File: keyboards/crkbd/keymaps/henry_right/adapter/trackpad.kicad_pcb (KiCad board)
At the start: 2 copper layers, 33.4 x 18.4 mm, 9 parts, among them J1 Conn_01x12, U1 Elite-C, U3 NCP1117-3.3_SOT223, U4 TXB0104D

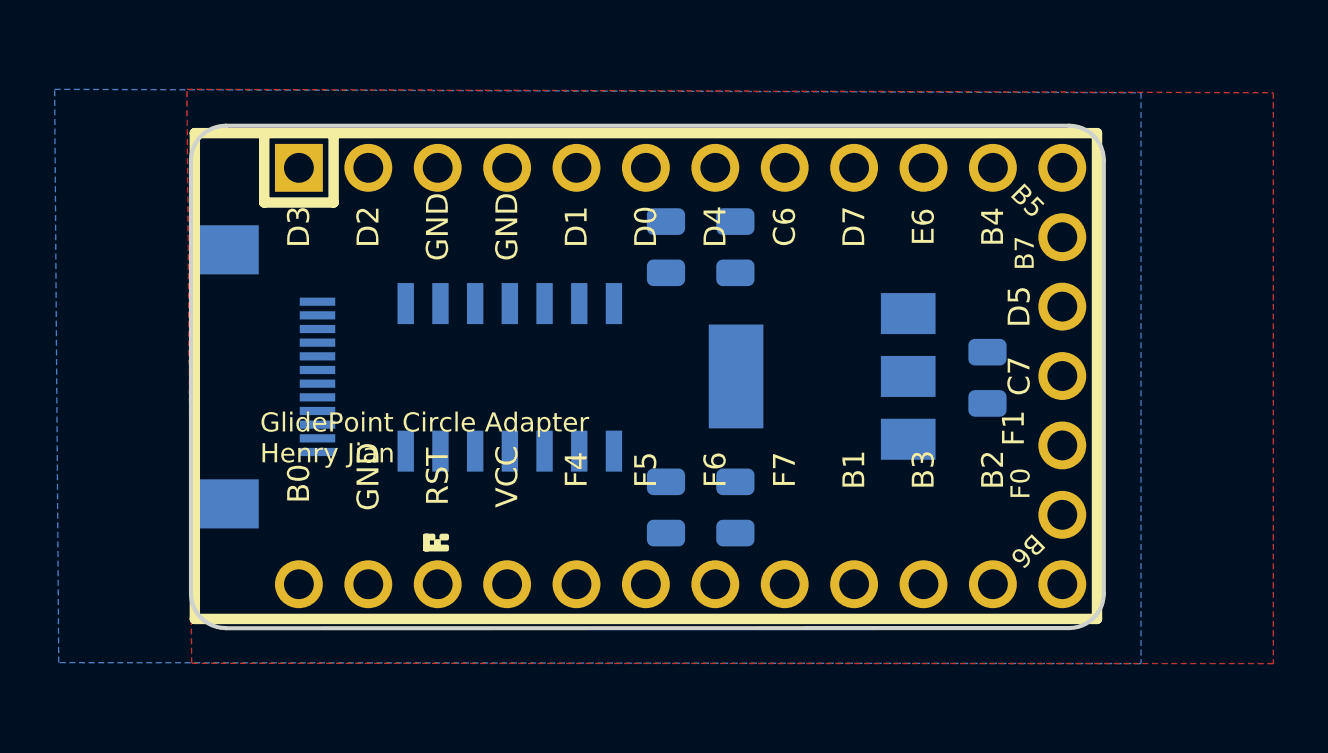
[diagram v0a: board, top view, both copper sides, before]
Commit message: 전체
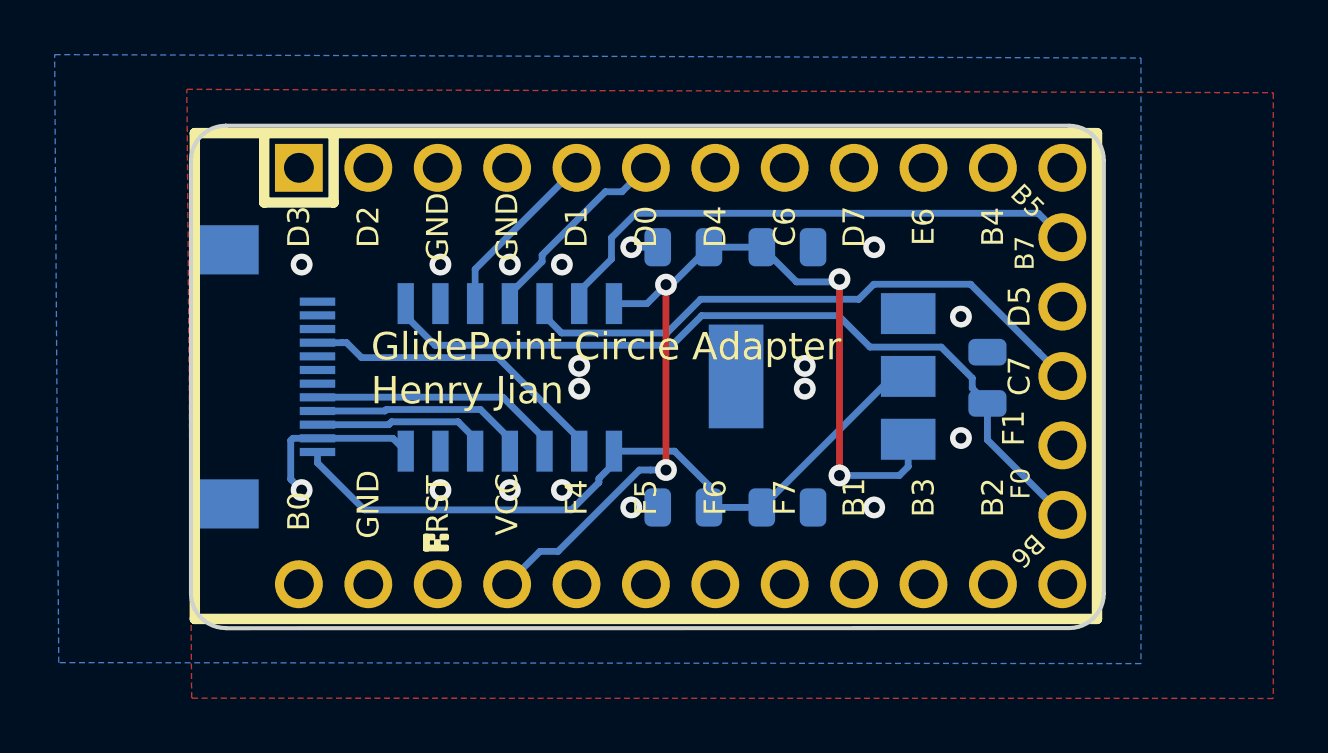
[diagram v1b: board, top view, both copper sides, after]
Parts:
- moved C1 1.91 mm to (119.4, 74.3), turned to 0 degrees
- moved C2 1.91 mm to (119.4, 83.8), turned to 0 degrees
- moved C3 0.63 mm to (115.6, 83.8), turned to 180 degrees
- moved C4 0.63 mm to (115.6, 74.3), turned to 180 degrees
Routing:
- net +5V: track 0.00 -> 34.8 mm, vias 0 -> 4
- net LVL_SHIFT: track 0.00 -> 29.4 mm
- net +3V3: track 0.00 -> 27.3 mm
- net TP_BTN1: track 0.00 -> 21.8 mm
- net TP_DR: track 0.00 -> 20.1 mm
- net TP_DR_3V3: track 0.00 -> 11.5 mm
- net TP_BTN1_3V3: track 0.00 -> 9.39 mm
- net TP_SCL_3V3: track 0.00 -> 7.96 mm
- net PD0: track 0.00 -> 7.39 mm
- net GND: track 0.00 -> 7.39 mm, vias 0 -> 18
- net TP_SDA_3V3: track 0.00 -> 6.52 mm
- net PD1: track 0.00 -> 6.51 mm
